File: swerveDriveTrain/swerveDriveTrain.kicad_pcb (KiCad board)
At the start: 4 copper layers, 87.2 x 48 mm, 8 parts, among them IC1 TCAN3414DR, J1 RJ45, J2 Screw_Terminal_01x02, J3 Conn_01x06_Pin, J4 S6B-PH-K-S_LF__SN_, P1 USB_C_Plug_USB2.0, U2 Teensy4.0

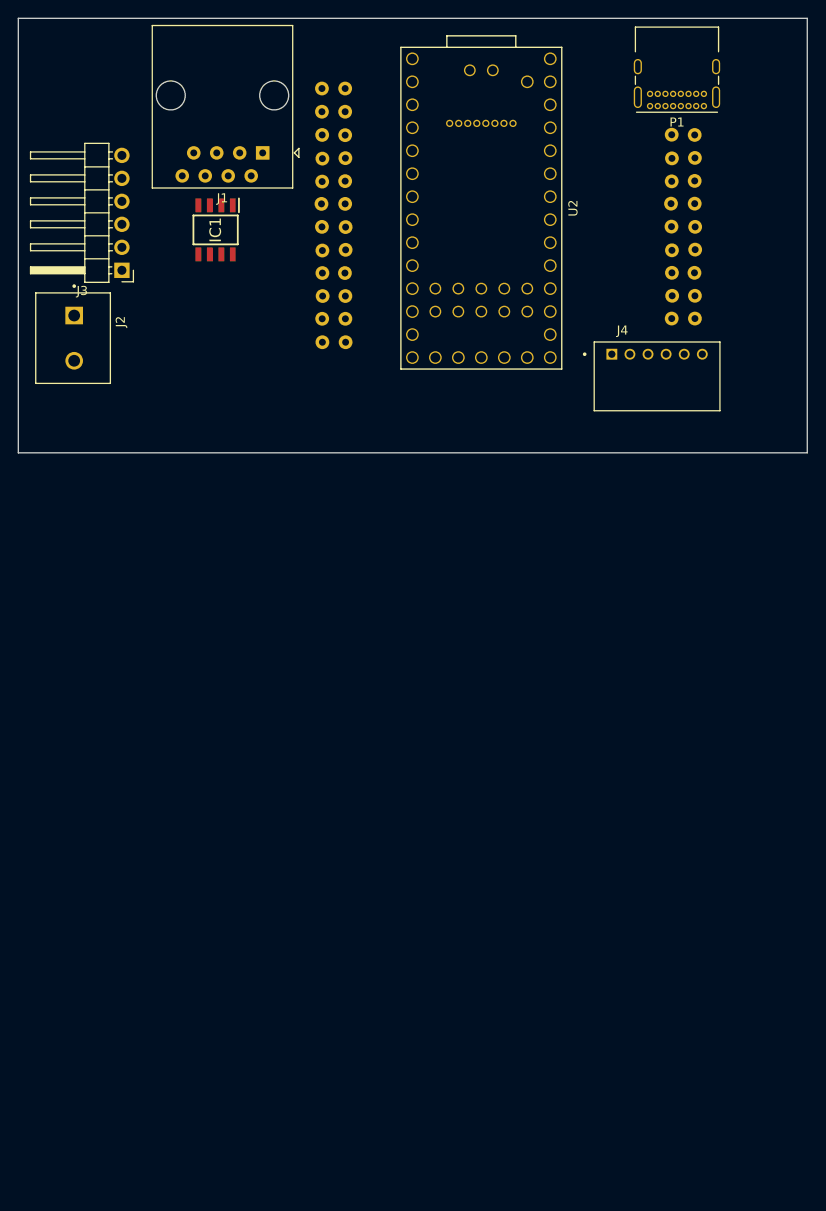
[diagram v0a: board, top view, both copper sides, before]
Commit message: work on the swerve drive
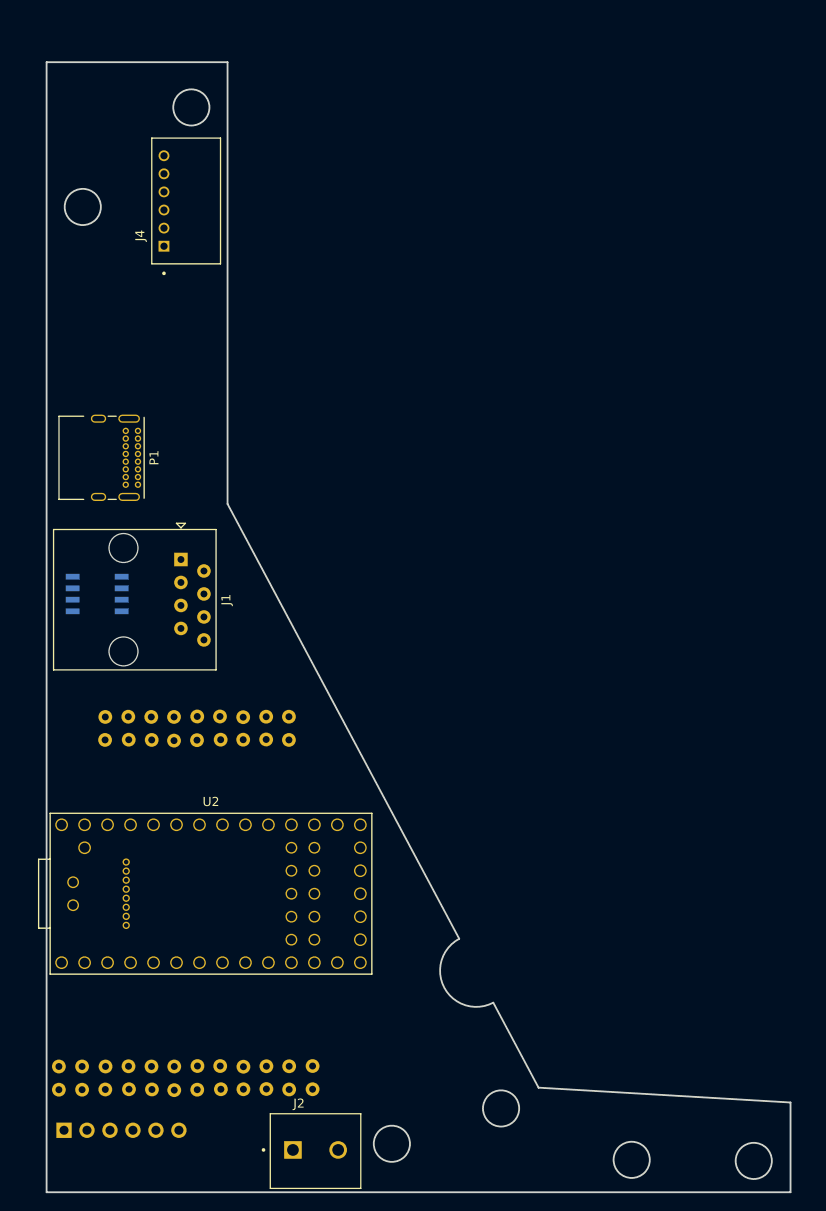
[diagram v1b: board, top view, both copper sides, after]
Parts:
- IC1, J3: moved to B.Cu
- moved J2 102.3 mm to (39.7, 140.5), turned to 0 degrees
- moved J3 95.3 mm to (16.9, 134.1), turned to -90 degrees
- moved U1 90.3 mm to (25.1, 107.4), turned to -90 degrees
- moved U2 81.4 mm to (33.1, 108.0), turned to 0 degrees
- moved P1 72.1 mm to (25.1, 56.8), turned to -90 degrees
- moved J4 57.1 mm to (27.9, 31.4), turned to 90 degrees
- moved J1 45.8 mm to (29.8, 71.0), turned to -90 degrees
- moved IC1 42.3 mm to (20.5, 74.8), turned to 0 degrees
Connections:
- J1 pad 4: CANP -> GND
- J1 pad 5: CANN -> GND
- J1 pad 7: GND -> CANP
- J1 pad 8: GND -> CANN
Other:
- board size 87.2 x 48 mm -> 82.2 x 124.9 mm
